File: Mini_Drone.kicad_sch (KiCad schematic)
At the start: 0 parts

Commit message: Motor Drivers no cap
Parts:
- added D1, D2, D3, D4: SS24, Diode_SMD:D_SMA, symbol Diode:SS24
- added Q1, Q2, Q3, Q4: AO3400A, Package_TO_SOT_SMD:SOT-23, symbol Transistor_FET:AO3400A
- added R1, R2, R3, R4: R, symbol Device:R
- added TP1, TP10, TP11, TP12, TP2, TP3, TP4, TP5, TP6, TP7, TP8, TP9: TestPoint, symbol Connector:TestPoint
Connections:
- new net: D4.2 (A), Q4.3 (D), TP12.1
- new net: D1.1 (K), TP1.1, TP2.1
- new net: D3.2 (A), Q3.3 (D), TP11.1
- new net: D2.1 (K), TP3.1, TP4.1
- new net: D2.2 (A), Q2.3 (D), TP10.1
- new net: D4.1 (K), TP7.1, TP8.1
- new net: D3.1 (K), TP5.1, TP6.1
- new net: D1.2 (A), Q1.3 (D), TP9.1
- new net GND: Q1.2 (S), Q2.2 (S), Q3.2 (S), Q4.2 (S), R1.2, R2.2, R3.2, R4.2
- new net GPIO: Q1.1 (G), Q2.1 (G), Q3.1 (G), Q4.1 (G), R1.1, R2.1, R3.1, R4.1

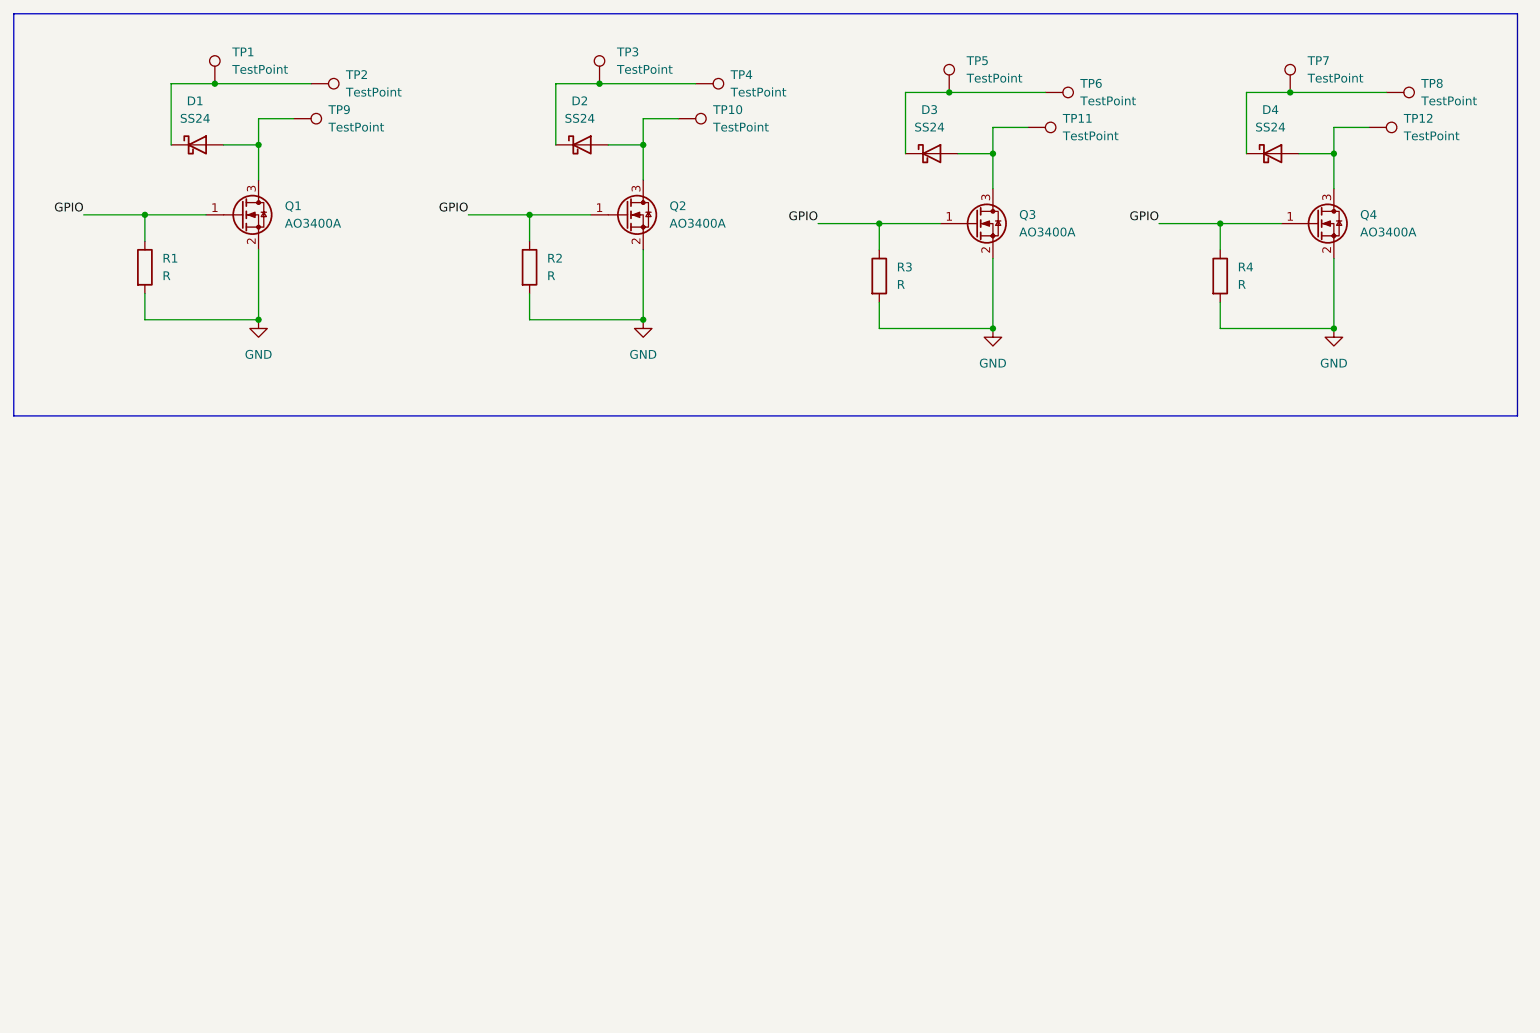
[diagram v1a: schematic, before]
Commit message: Version 1
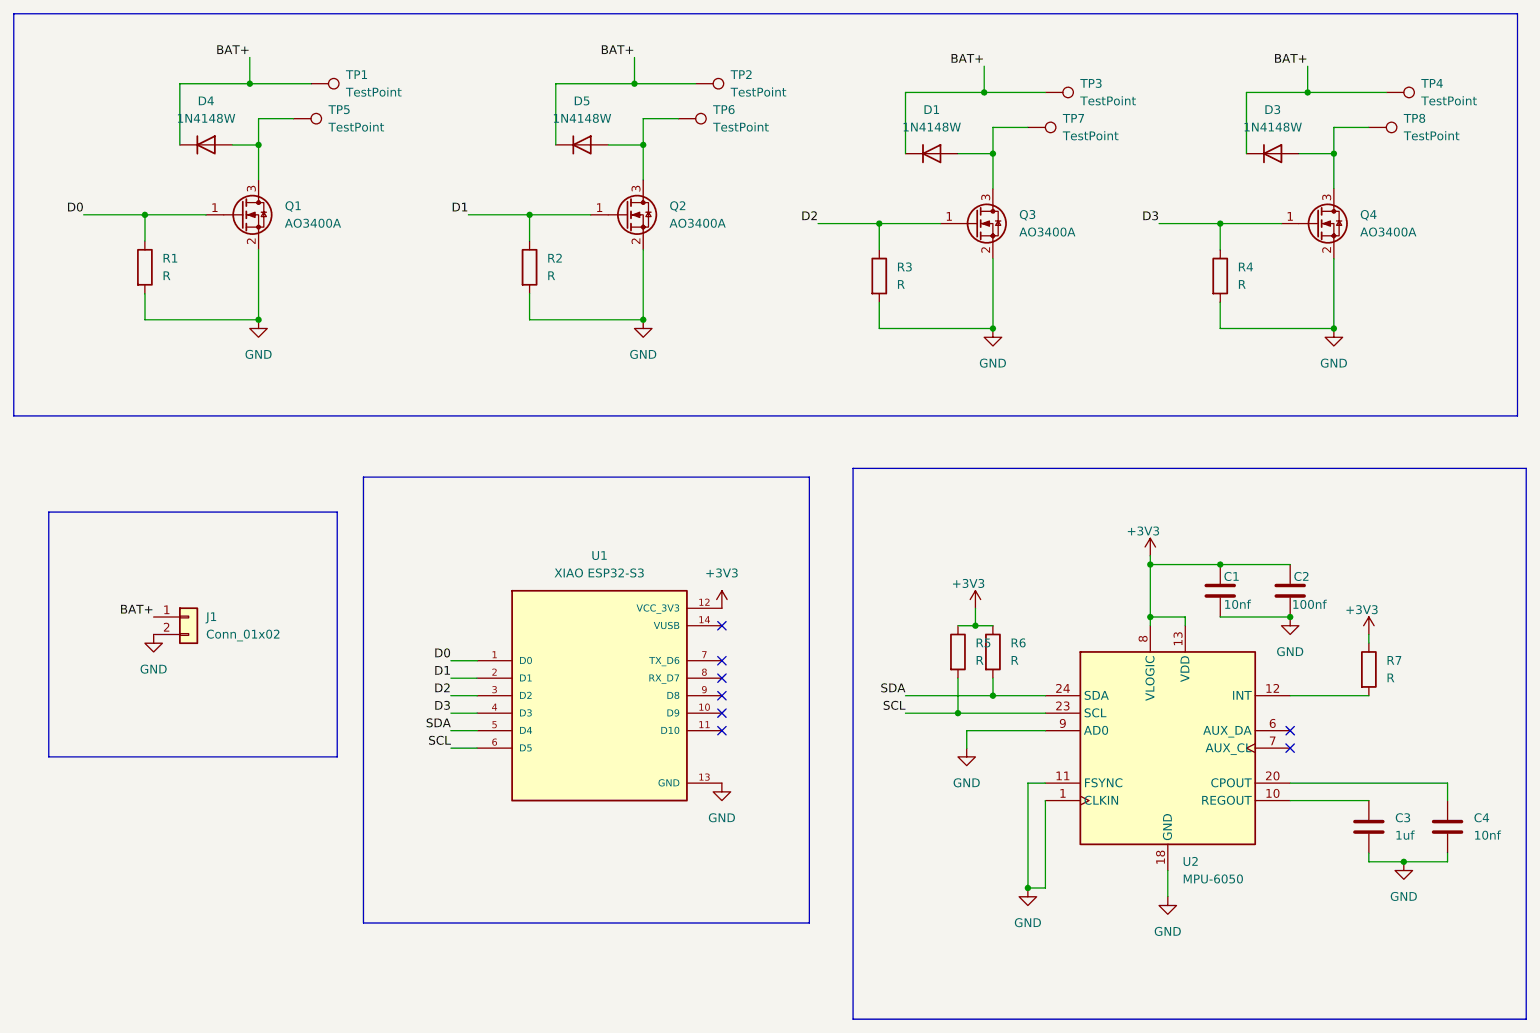
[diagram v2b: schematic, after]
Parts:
- removed D1, D2, D3, D4: SS24, Diode_SMD:D_SMA, symbol Diode:SS24
- removed TP1, TP3, TP5, TP7: TestPoint, symbol Connector:TestPoint
- added C1, C4: 10nf, Capacitor_SMD:C_0201_0603Metric_Pad0.64x0.40mm_HandSolder, symbol Device:C
- added C2: 100nf, Capacitor_SMD:C_0201_0603Metric_Pad0.64x0.40mm_HandSolder, symbol Device:C
- added C3: 1uf, Capacitor_SMD:C_0201_0603Metric_Pad0.64x0.40mm_HandSolder, symbol Device:C
- added D1, D3, D4, D5: 1N4148W, Diode_SMD:D_SOD-123, symbol Diode:1N4148W
- added J1: Conn_01x02, Connector_JST:JST_EH_S2B-EH_1x02_P2.50mm_Horizontal, symbol Connector_Generic:Conn_01x02
- added R5, R6, R7: R, Resistor_SMD:R_0201_0603Metric_Pad0.64x0.40mm_HandSolder, symbol Device:R
- added U1: XIAO ESP32-S3, Drone_prj:XIAO ESP32-S3, symbol Drone_prj:XIAO ESP32-S3
- added U2: MPU-6050, Sensor_Motion:InvenSense_QFN-24_4x4mm_P0.5mm, symbol Sensor_Motion:MPU-6050
- R1, R2, R3, R4: footprint (none) -> Resistor_SMD:R_0201_0603Metric_Pad0.64x0.40mm_HandSolder
- TP1: renamed from TP2; footprint (none) -> TestPoint:TestPoint_Pad_1.5x1.5mm
- TP2: renamed from TP4; footprint (none) -> TestPoint:TestPoint_Pad_1.5x1.5mm
- TP3: renamed from TP6; footprint (none) -> TestPoint:TestPoint_Pad_1.5x1.5mm
- TP4: renamed from TP8; footprint (none) -> TestPoint:TestPoint_Pad_1.5x1.5mm
- TP5: renamed from TP9; footprint (none) -> TestPoint:TestPoint_Pad_1.5x1.5mm
- TP6: renamed from TP10; footprint (none) -> TestPoint:TestPoint_Pad_1.5x1.5mm
- TP7: renamed from TP11; footprint (none) -> TestPoint:TestPoint_Pad_1.5x1.5mm
- TP8: renamed from TP12; footprint (none) -> TestPoint:TestPoint_Pad_1.5x1.5mm
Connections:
- net GND: now also C1.2, C2.2, C3.2, C4.2, J1.2 (Pin_2), U1.13 (GND), U2.1 (CLKIN), U2.11 (FSYNC), U2.18 (GND), U2.9 (AD0)
- net at Q4.3 (D), TP8.1: now also D3.2 (A)
- net BAT+: now reaches TP1.1
- net BAT+: now also TP2.1, TP3.1, TP4.1, D1.1 (K), D3.1 (K), D4.1 (K), D5.1 (K), J1.1 (Pin_1)
- net at Q3.3 (D), TP7.1: now also D1.2 (A)
- net at Q2.3 (D), TP6.1: now also D5.2 (A)
- net at Q1.3 (D), TP5.1: now also D4.2 (A)
- removed net GPIO: Q1.1 (G), Q2.1 (G), Q3.1 (G), Q4.1 (G), R1.1, R2.1, R3.1, R4.1
- new net: C3.1, U2.10 (REGOUT)
- new net: R7.2, U2.12 (INT)
- new net: C4.1, U2.20 (CPOUT)
- new net +3V3: C1.1, C2.1, R5.1, R6.1, R7.1, U1.12 (VCC_3V3), U2.13 (VDD), U2.8 (VLOGIC)
- new net D0: Q1.1 (G), R1.1, U1.1 (D0)
- new net D1: Q2.1 (G), R2.1, U1.2 (D1)
- new net D2: Q3.1 (G), R3.1, U1.3 (D2)
- new net D3: Q4.1 (G), R4.1, U1.4 (D3)
- new net SCL: R5.2, U1.6 (D5), U2.23 (SCL)
- new net SDA: R6.2, U1.5 (D4), U2.24 (SDA)
- no-connect marks 0 -> 8
